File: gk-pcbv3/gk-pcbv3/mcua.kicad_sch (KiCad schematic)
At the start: 19 parts, among them J12 Conn_01x03, SW1 SW_Push, U4 STM32H7S7L8H6H, Y2 32.768kHz R26-32.768-12.5

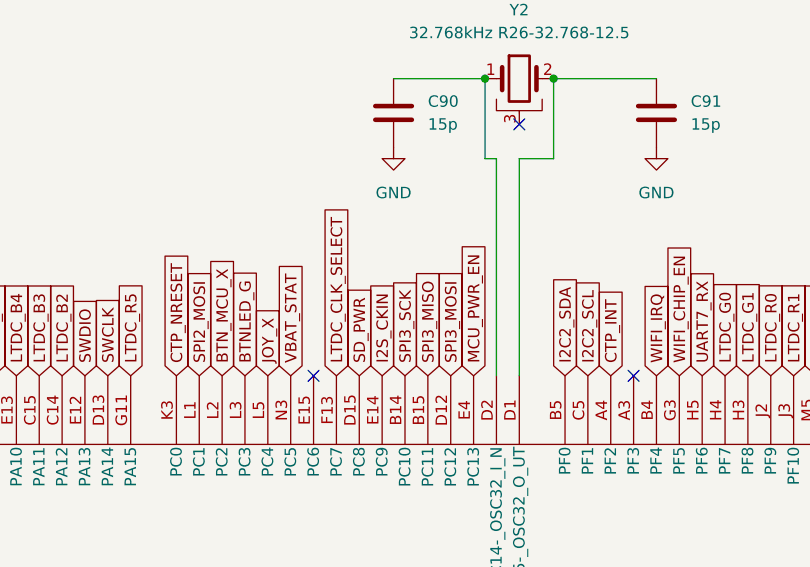
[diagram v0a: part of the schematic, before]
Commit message: gerbers for v3.1
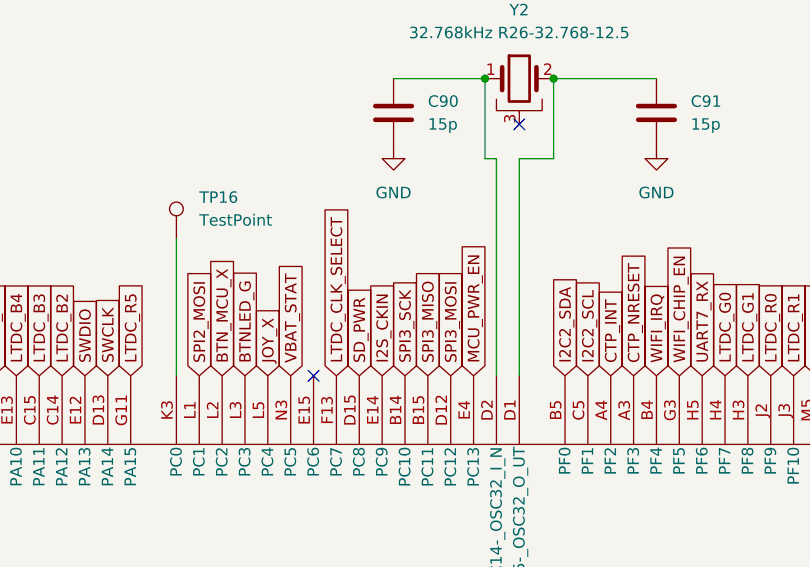
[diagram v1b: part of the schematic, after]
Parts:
- added TP16: TestPoint, Connector_PinHeader_2.54mm:PinHeader_1x01_P2.54mm_Vertical, symbol Connector:TestPoint
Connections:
- net CTP_NRESET: now also U4.A3 (PF3); no longer U4.K3 (PC0)
- new net: TP16.1, U4.K3 (PC0)
- no-connect marks 4 -> 3
